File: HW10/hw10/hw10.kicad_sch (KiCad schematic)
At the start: 30 parts, among them J1 Screw_Terminal_01x02, J2 Screw_Terminal_01x02, Q1 BC807, Q2 BC817, Q3 IRLZ44N, U1 LM317_TO-220, U2 NE555P

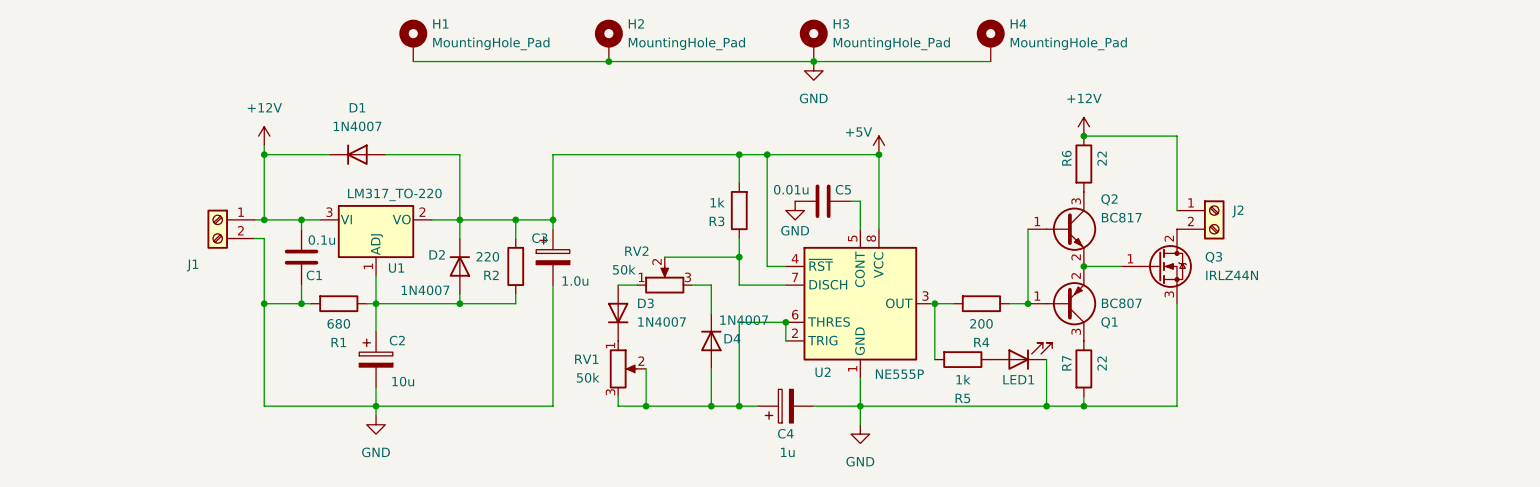
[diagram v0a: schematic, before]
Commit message: HW10 done
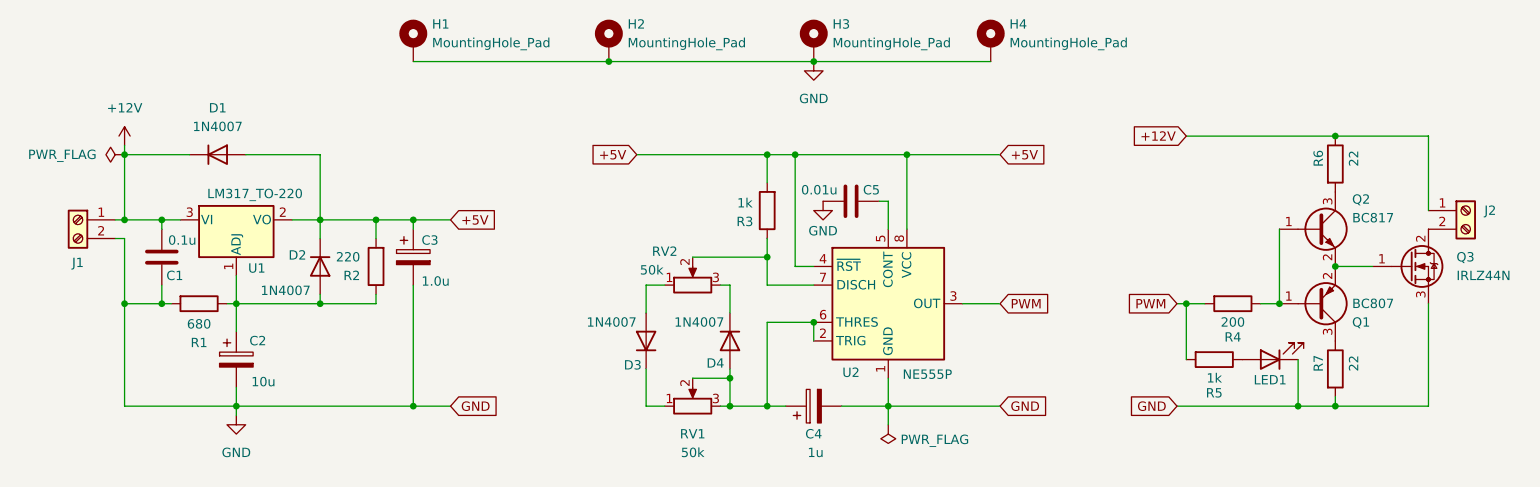
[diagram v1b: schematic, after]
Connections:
- net PWM: now reaches R4.2, R5.2, U2.3 (OUT)
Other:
- moved on the sheet: C1, C2, C3, C4, C5, D1, D2, D3, D4, J1, J2, LED1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
